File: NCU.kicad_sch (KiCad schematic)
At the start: 4 parts, among them J1 RJ45, J2 USB_B, J3 Micro_SD_Card, J4 USB_C_Receptacle

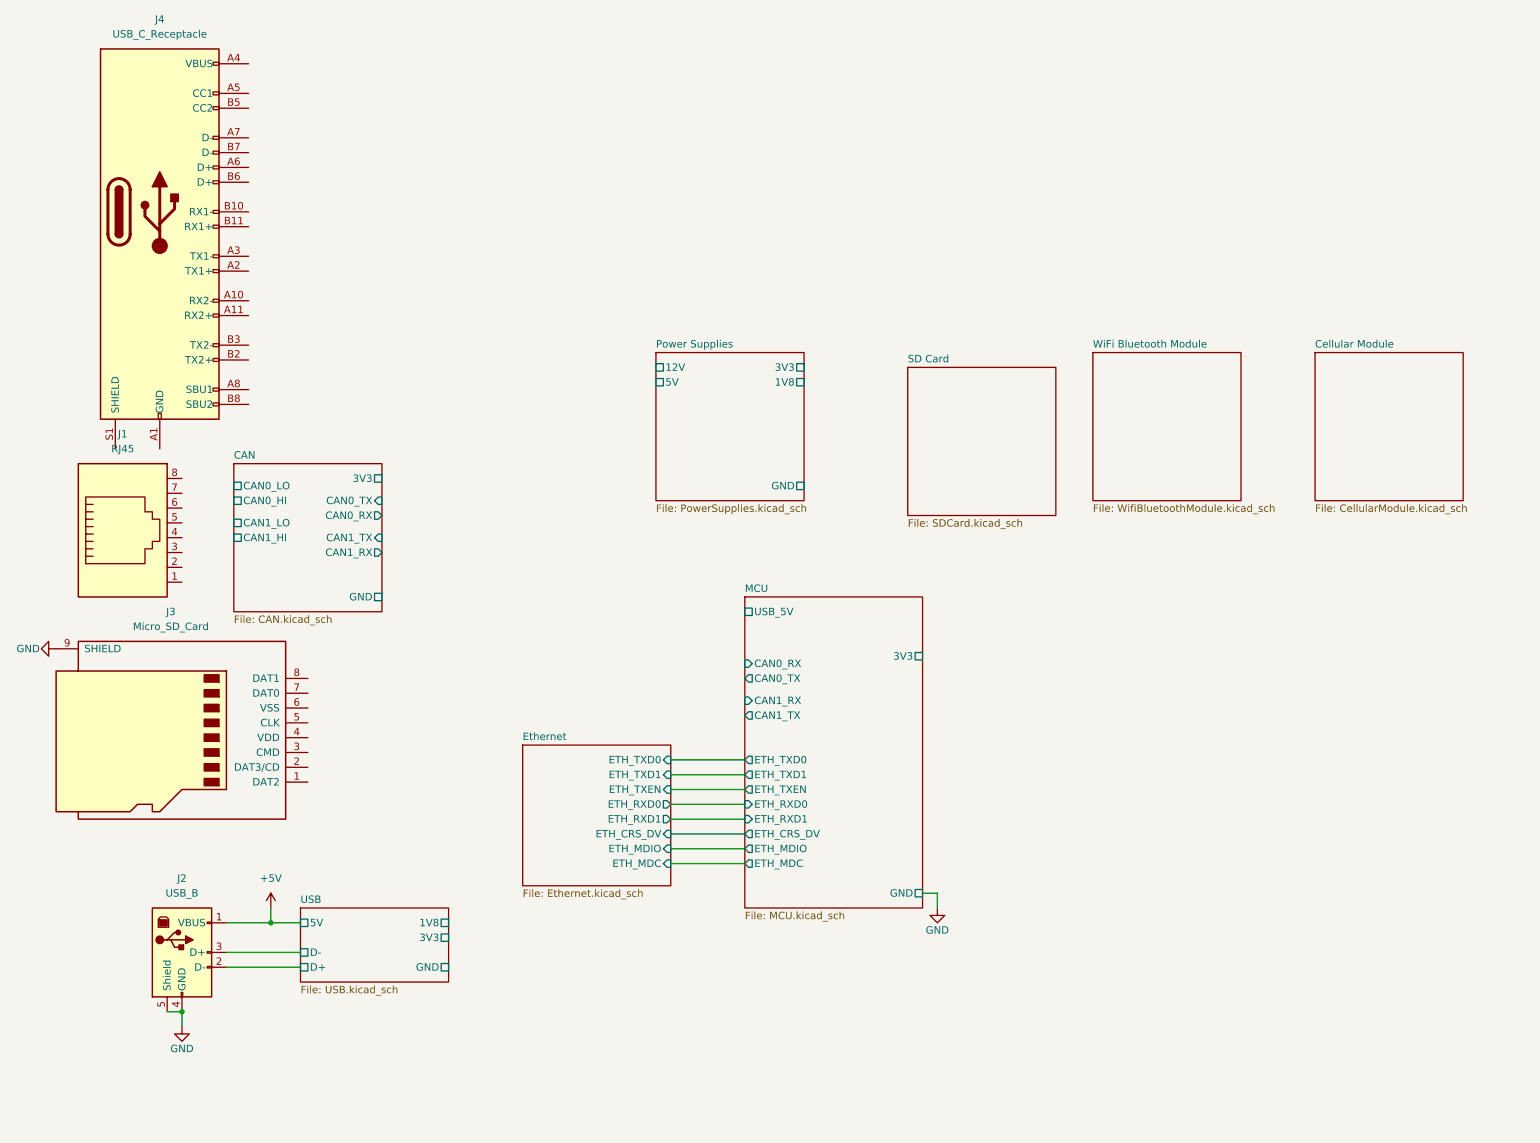
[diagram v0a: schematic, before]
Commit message: wip
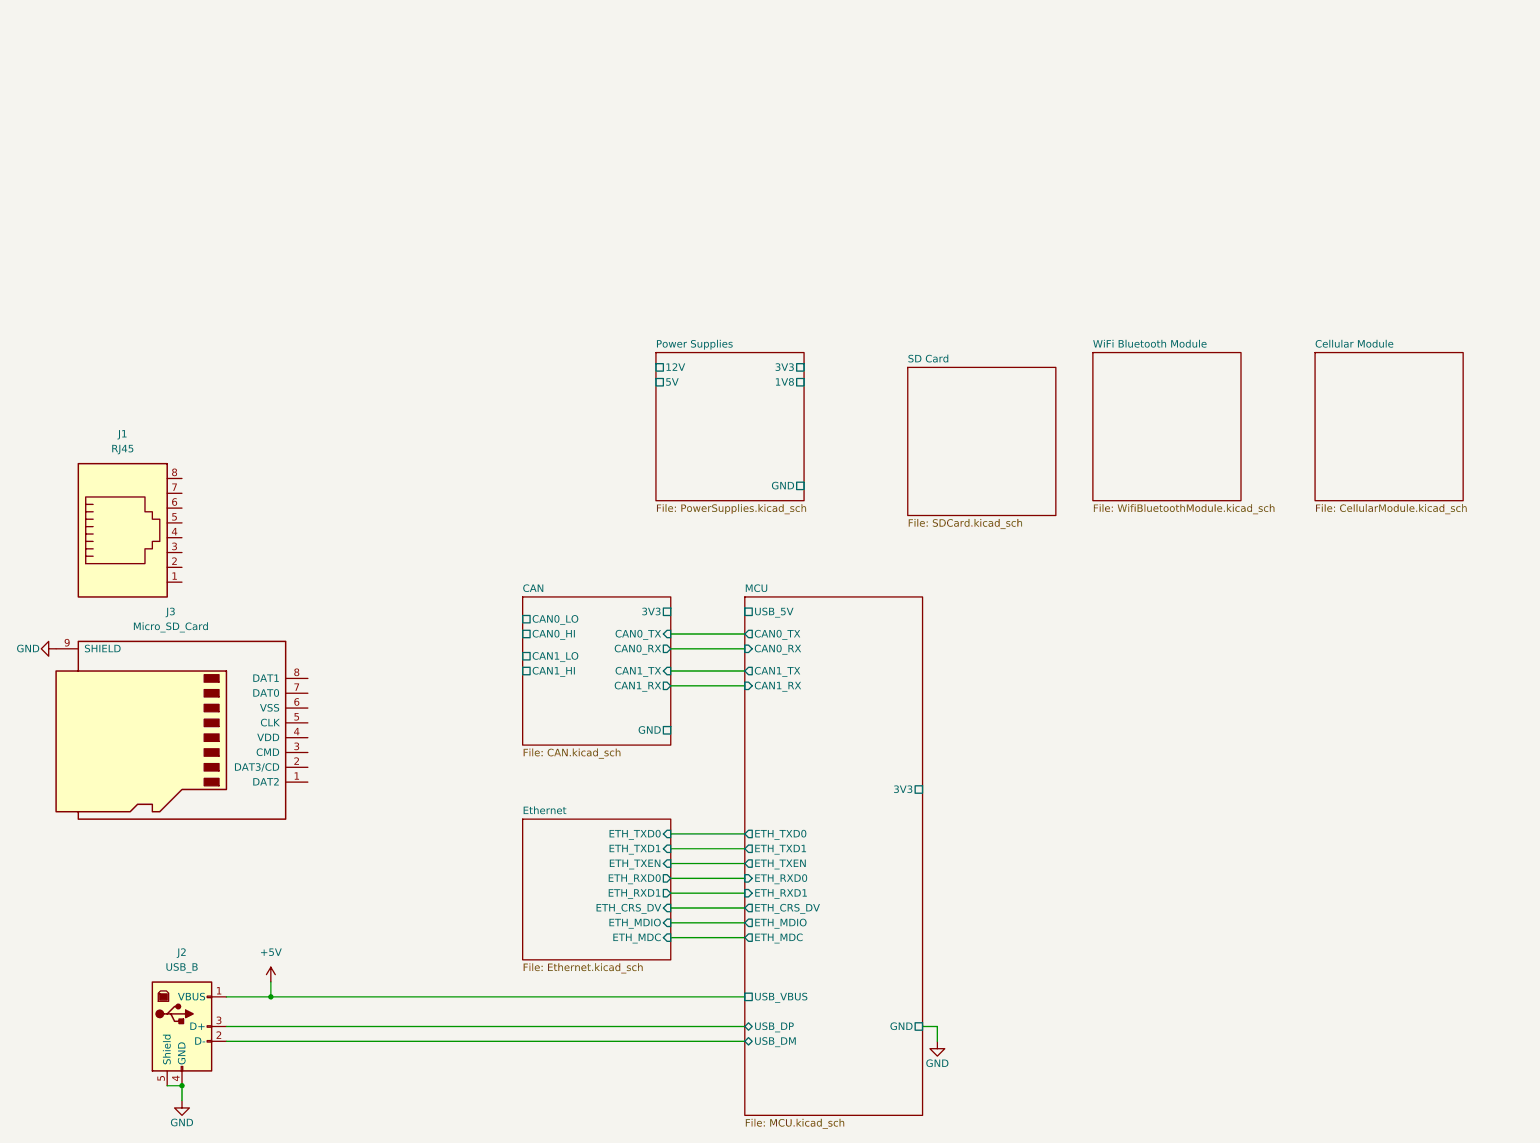
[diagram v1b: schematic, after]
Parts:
- removed J4: USB_C_Receptacle, symbol Connector:USB_C_Receptacle
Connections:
- net USB/D+ renamed MCU/USB_DM
- net USB/D- renamed MCU/USB_DP
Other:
- removed sheet USB
- sheet MCU ports: added USB_DM, USB_DP, USB_VBUS; removed none
- moved on the sheet: J2
